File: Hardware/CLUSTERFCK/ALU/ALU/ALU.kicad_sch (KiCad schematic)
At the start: 30 parts, among them U1 74LS86, U10 74LS08, U2 74LS86, U3 74LS245, U4 74LS283, U5 74LS283, U8 74LS02

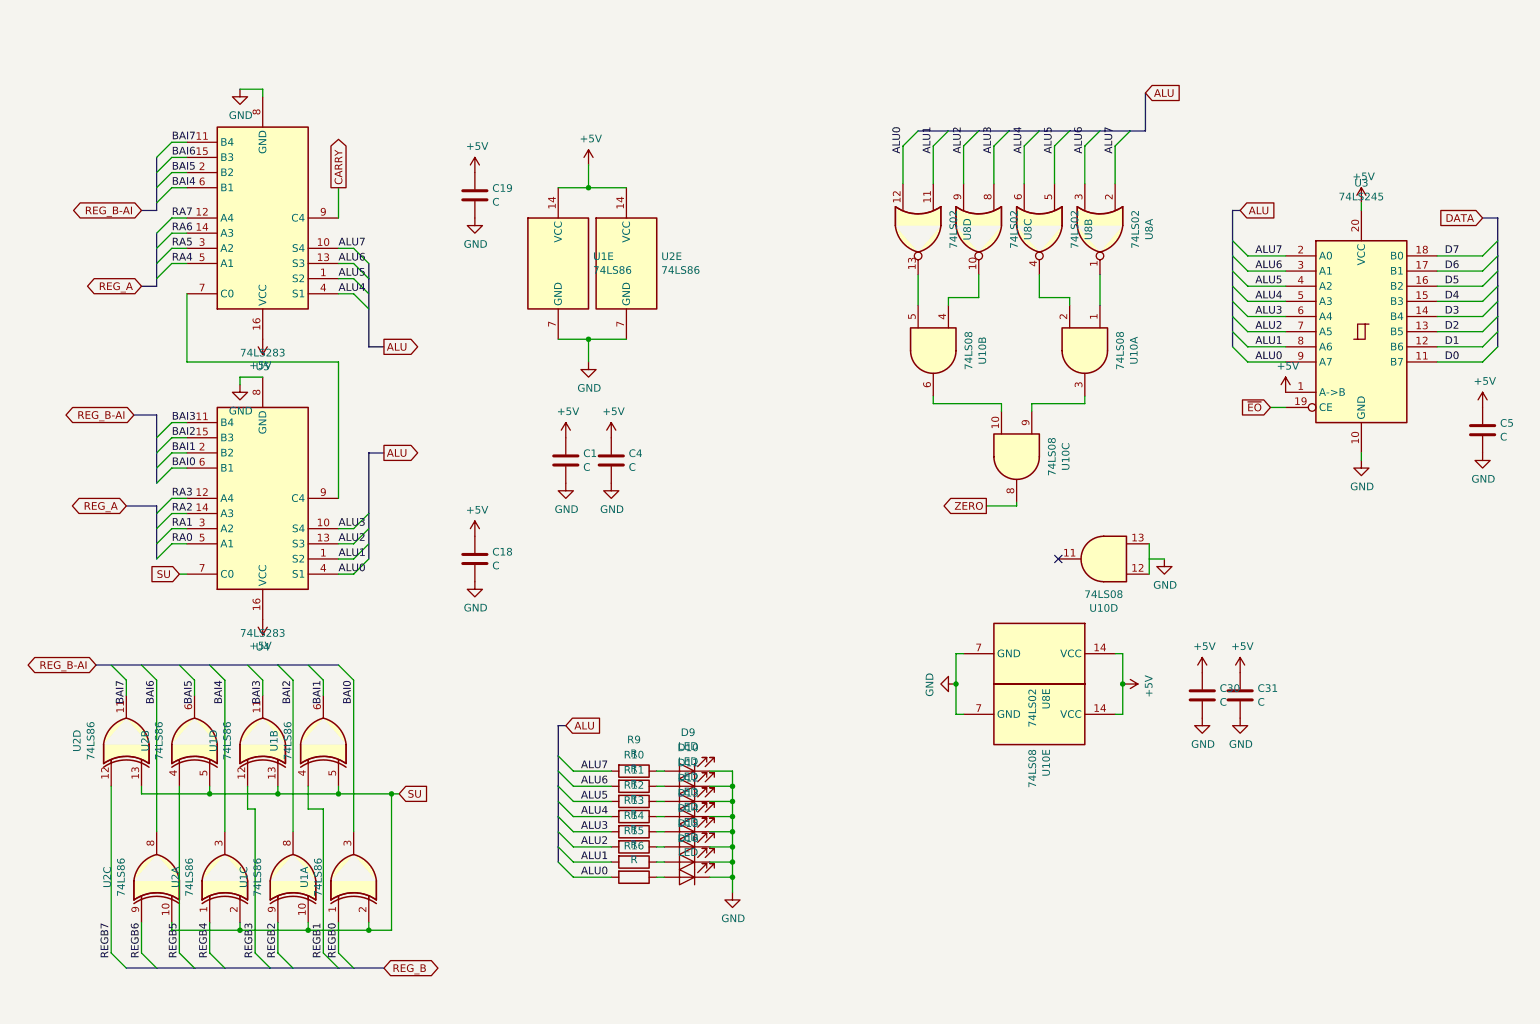
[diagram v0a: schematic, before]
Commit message: unstable switching device push
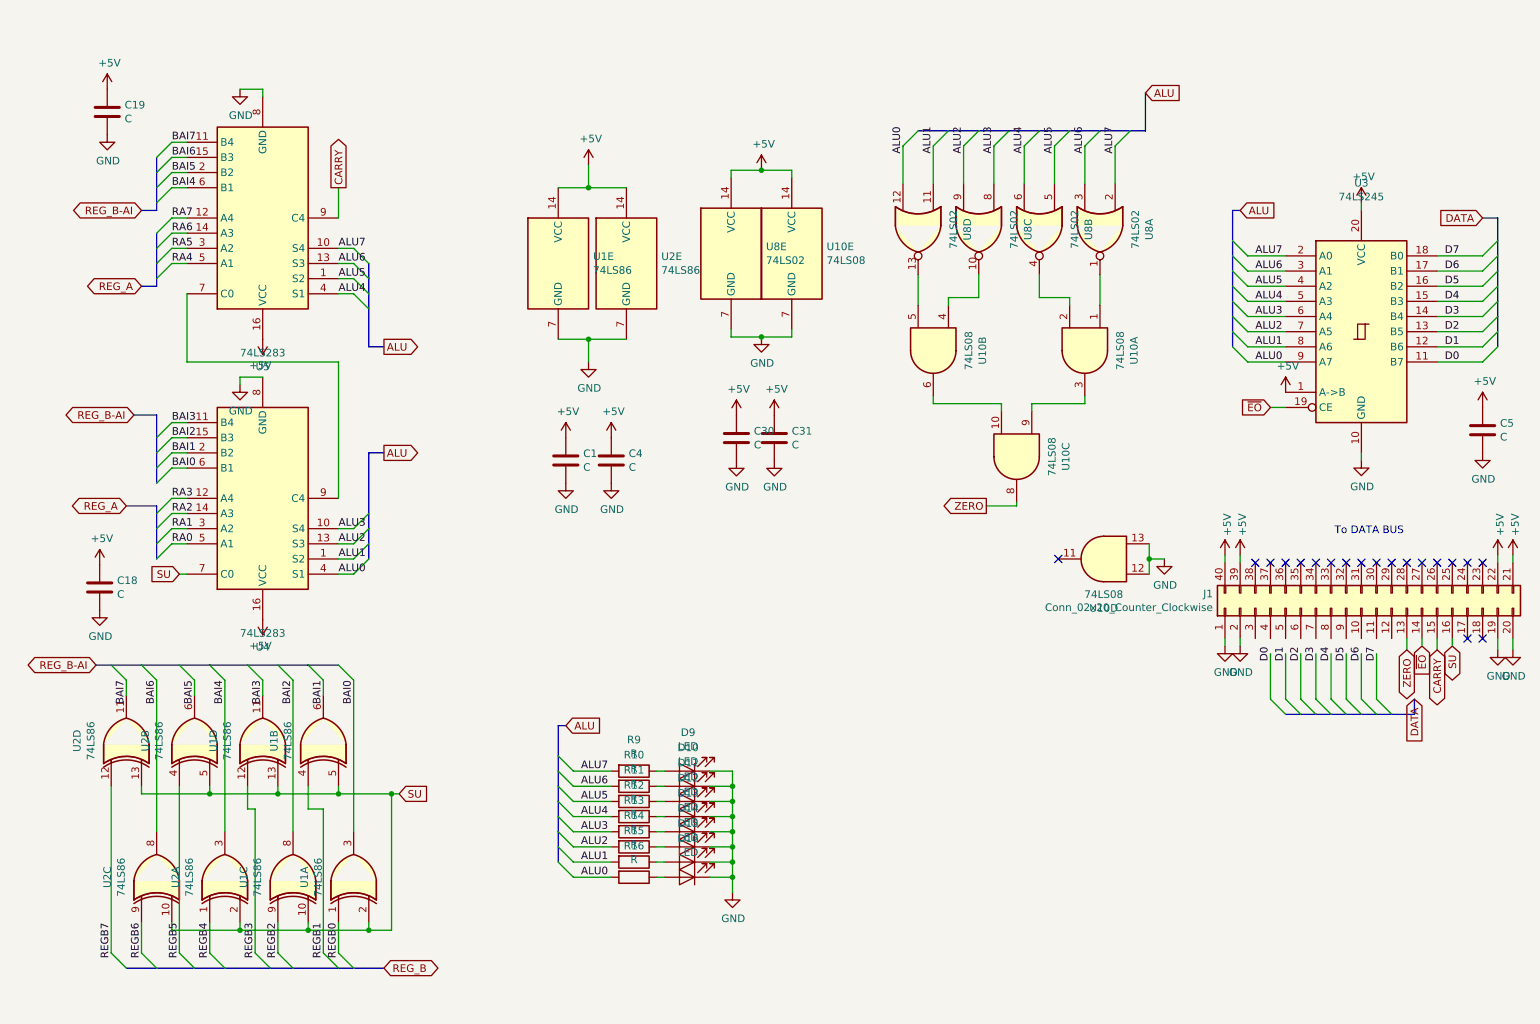
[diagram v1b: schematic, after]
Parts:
- added J1: Conn_02x20_Counter_Clockwise, Connector_PinSocket_2.54mm:PinSocket_2x20_P2.54mm_Horizontal, symbol Connector_Generic:Conn_02x20_Counter_Clockwise
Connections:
- net +5V: now also J1.21 (Pin_21), J1.22 (Pin_22), J1.39 (Pin_39), J1.40 (Pin_40)
- net CARRY: now also J1.15 (Pin_15)
- net GND: now also U10.12, U10.13, J1.1 (Pin_1), J1.19 (Pin_19), J1.2 (Pin_2), J1.20 (Pin_20)
- net SU: now also J1.16 (Pin_16)
- net ZERO: now also J1.13 (Pin_13)
- net ~EO: now also J1.14 (Pin_14)
- no-connect marks 1 -> 19
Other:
- note added: "To DATA BUS"
- moved on the sheet: C18, C19, C30, C31, U10E, U8E

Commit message: temporary unstable push
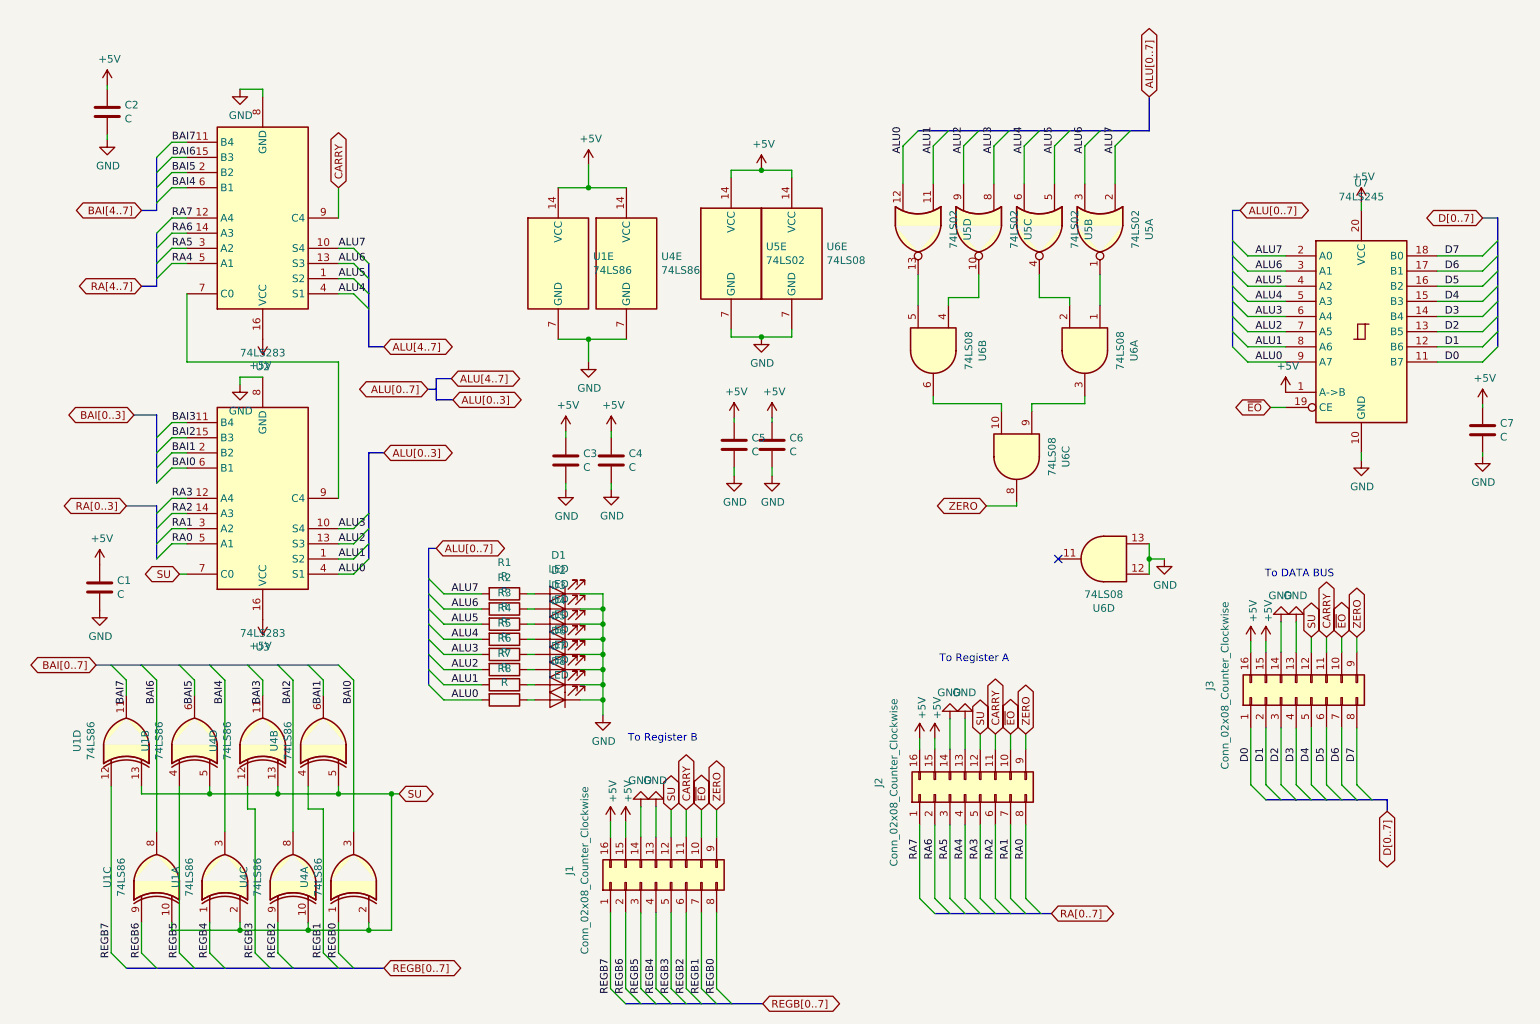
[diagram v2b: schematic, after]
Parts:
- removed J1: Conn_02x20_Counter_Clockwise, Connector_PinSocket_2.54mm:PinSocket_2x20_P2.54mm_Horizontal, symbol Connector_Generic:Conn_02x20_Counter_Clockwise
- added J1, J2, J3: Conn_02x08_Counter_Clockwise, symbol Connector_Generic:Conn_02x08_Counter_Clockwise
- U2: renamed from U5; footprint Package_DIP:DIP-16_W7.62mm_Socket_LongPads -> Package_SO:SOIC-16W_5.3x10.2mm_P1.27mm
- U3: renamed from U4; footprint Package_DIP:DIP-16_W7.62mm_Socket_LongPads -> Package_SO:SOIC-16W_5.3x10.2mm_P1.27mm
- U5: renamed from U8; footprint Package_DIP:DIP-14_W7.62mm_Socket_LongPads -> Package_SO:SOIC-14_3.9x8.7mm_P1.27mm
- U6: renamed from U10; footprint Package_DIP:DIP-14_W7.62mm_Socket_LongPads -> Package_SO:SOIC-14_3.9x8.7mm_P1.27mm
- U7: renamed from U3; footprint Package_DIP:DIP-20_W7.62mm_Socket_LongPads -> Package_SO:SOIC-20W_7.5x12.8mm_P1.27mm
- renumbered C18 to C1, C19 to C2, C1 to C3, C30 to C5, C31 to C6, C5 to C7, D9 to D1, D10 to D2, D11 to D3, D12 to D4, D13 to D5, D14 to D6, D15 to D7, D16 to D8, R9 to R1, R10 to R2, R11 to R3, R12 to R4, R13 to R5, R14 to R6, R15 to R7, R16 to R8, U2 to U1, U1 to U4, U2 to U4
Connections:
- net +5V: now also J1.15 (Pin_15), J1.16 (Pin_16), J2.15 (Pin_15), J2.16 (Pin_16), J3.15 (Pin_15), J3.16 (Pin_16)
- net CARRY: now also J1.11 (Pin_11), J2.11 (Pin_11), J3.11 (Pin_11)
- net D0: now also J3.1 (Pin_1)
- net D1: now also J3.2 (Pin_2)
- net D2: now also J3.3 (Pin_3)
- net D3: now also J3.4 (Pin_4)
- net D4: now also J3.5 (Pin_5)
- net D5: now also J3.6 (Pin_6)
- net D6: now also J3.7 (Pin_7)
- net D7: now also J3.8 (Pin_8)
- net GND: now also J1.13 (Pin_13), J1.14 (Pin_14), J2.13 (Pin_13), J2.14 (Pin_14), J3.13 (Pin_13), J3.14 (Pin_14)
- net RA0: now also J2.8 (Pin_8)
- net RA1: now also J2.7 (Pin_7)
- net RA2: now also J2.6 (Pin_6)
- net RA3: now also J2.5 (Pin_5)
- net RA4: now also J2.4 (Pin_4)
- net RA5: now also J2.3 (Pin_3)
- net RA6: now also J2.2 (Pin_2)
- net RA7: now also J2.1 (Pin_1)
- net REGB0: now also J1.8 (Pin_8)
- net REGB1: now also J1.7 (Pin_7)
- net REGB2: now also J1.6 (Pin_6)
- net REGB3: now also J1.5 (Pin_5)
- net REGB4: now also J1.4 (Pin_4)
- net REGB5: now also J1.3 (Pin_3)
- net REGB6: now also J1.2 (Pin_2)
- net REGB7: now also J1.1 (Pin_1)
- net SU: now also J1.12 (Pin_12), J2.12 (Pin_12), J3.12 (Pin_12)
- net ZERO: now also J1.9 (Pin_9), J2.9 (Pin_9), J3.9 (Pin_9)
- net ~EO: now also J1.10 (Pin_10), J2.10 (Pin_10), J3.10 (Pin_10)
- no-connect marks 19 -> 1
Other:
- note added: "To Register A"
- note added: "To Register B"
- moved on the sheet: C5, C6, D1, D2, D3, D4, D5, D6, D7, D8, R1, R2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
